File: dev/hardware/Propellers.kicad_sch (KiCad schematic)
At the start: 17 parts, among them J201 CPU PGMR, J202 SPARE CPU HDR, J203 GPU PGMR, J204 SPARE GPU HDR, SW201 CPU ~{RES}, SW202 DEBUG, SW203 GPU ~{RES}

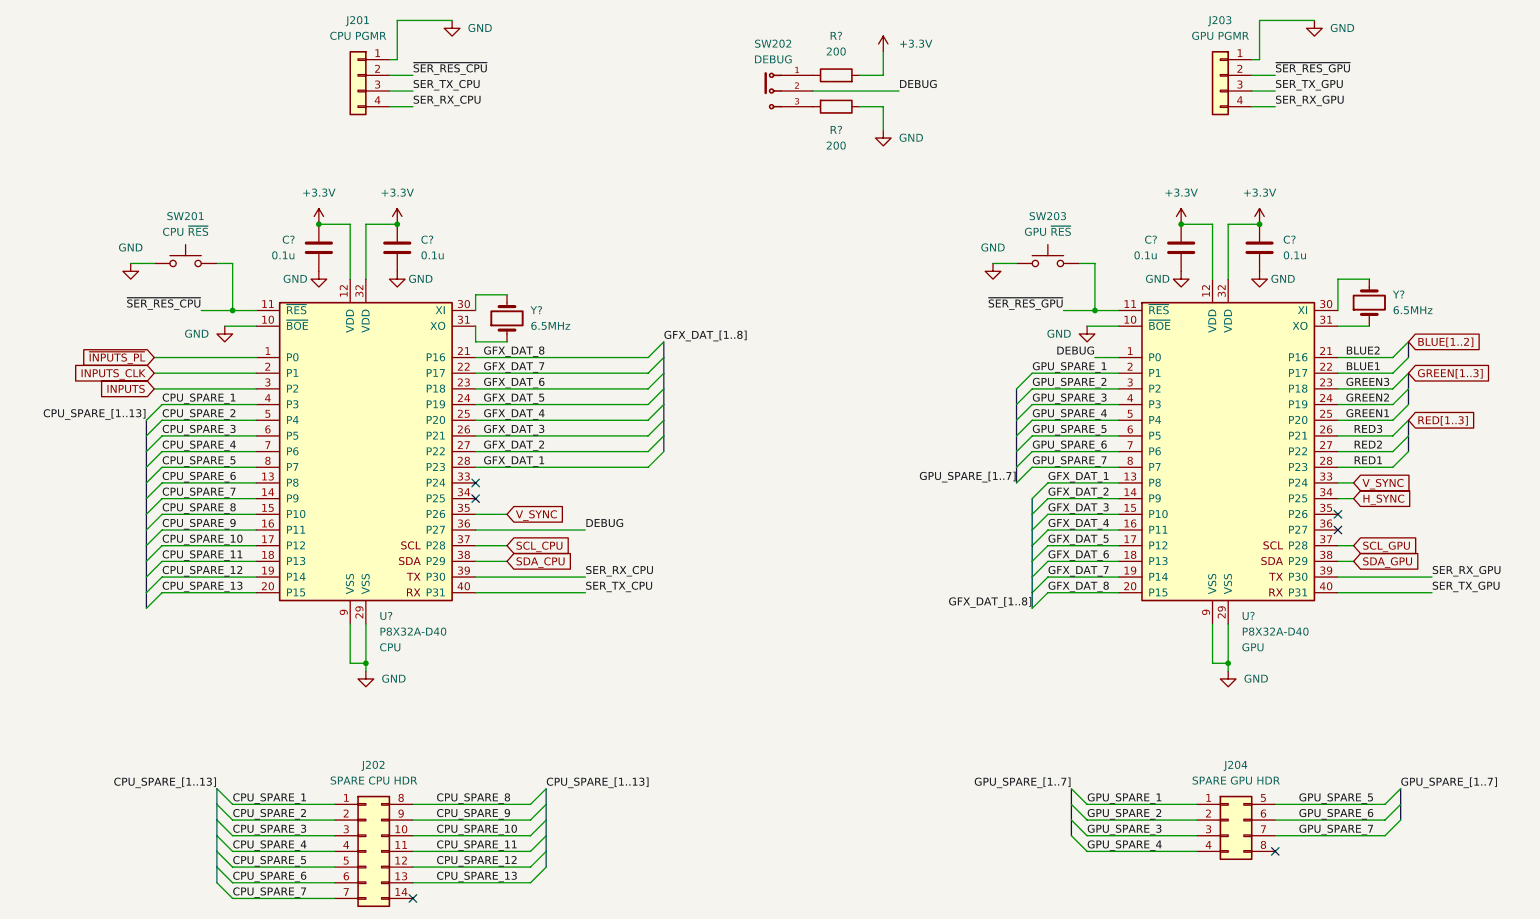
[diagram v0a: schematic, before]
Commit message: Finalized dev board administrivia
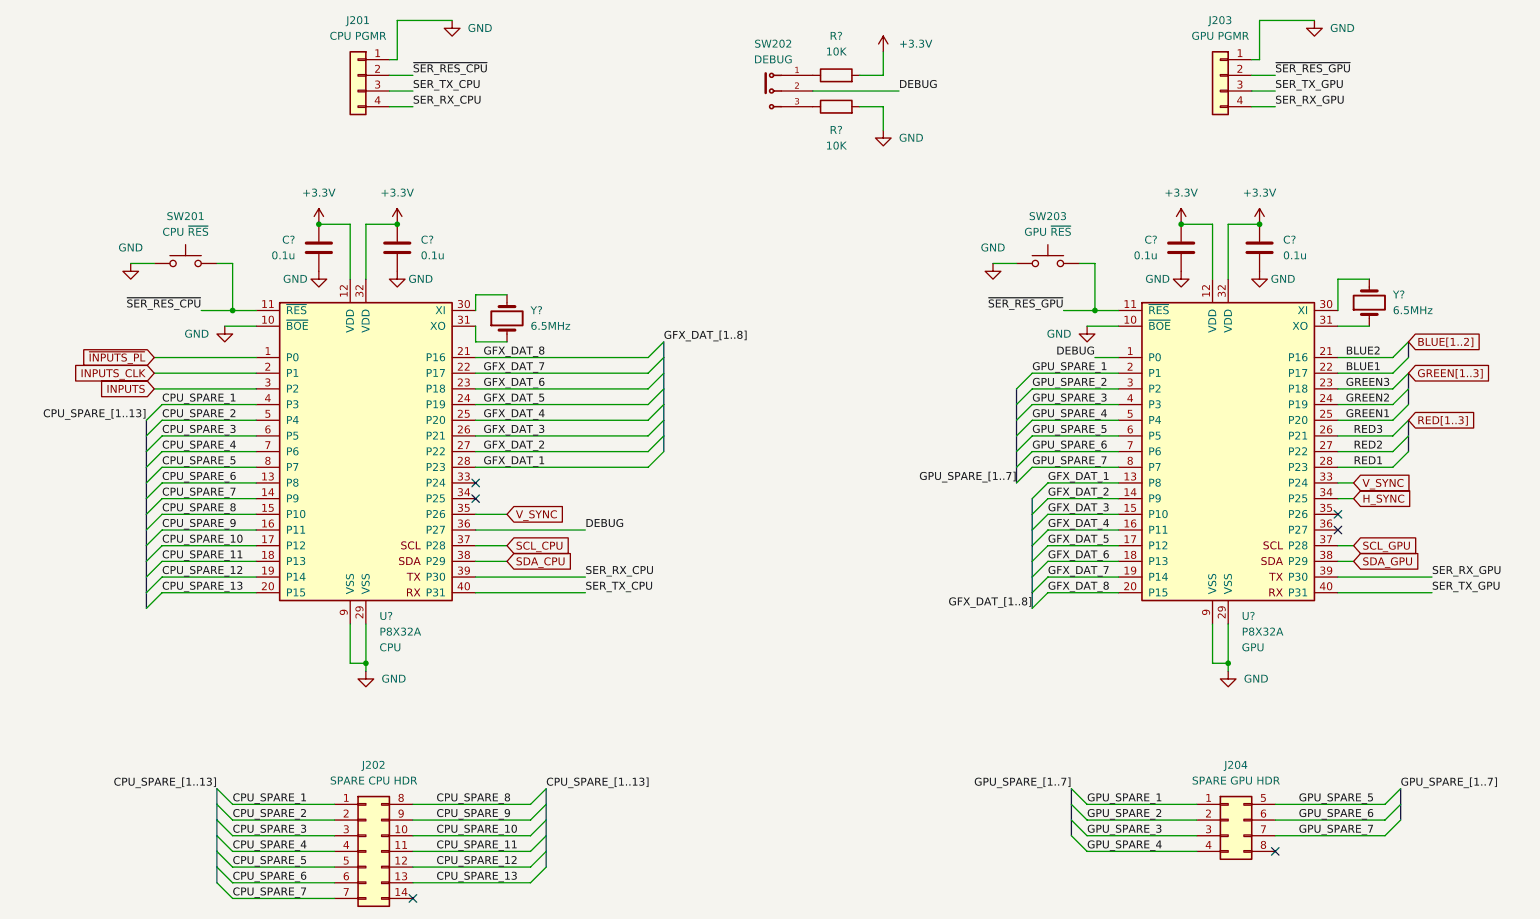
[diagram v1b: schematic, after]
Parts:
- removed C? (x3): 0.1u, Capacitor_THT:C_Disc_D3.4mm_W2.1mm_P2.50mm, symbol Device:C
- removed R?: 200, Resistor_THT:R_Axial_DIN0207_L6.3mm_D2.5mm_P10.16mm_Horizontal, symbol Device:R
- removed Y?: 6.5MHz, Crystal:Crystal_HC49-U_Vertical, symbol Device:Crystal
- added C? (x3): 0.1u, Capacitor_THT:C_Disc_D3.4mm_W2.1mm_P2.50mm, symbol Device:C
- added R?: 10K, Resistor_THT:R_Axial_DIN0207_L6.3mm_D2.5mm_P10.16mm_Horizontal, symbol Device:R
- added Y?: 6.5MHz, Crystal:Crystal_HC49-U_Vertical, symbol Device:Crystal
- C?, J201, J203: Part (none) -> K104K15X7RF5TL2
- J202: Part (none) -> PH2-14-UA
- J204: Part (none) -> PH2-08-UA
- R?: value 200 -> 10K; Part (none) -> RNF14FTD10K0
- SW201, SW203: Part (none) -> B3F-1002
- SW202: Part (none) -> EG1218
- U? (x2): value P8X32A-D40 -> P8X32A; Part (none) -> P8X32A-D40
- Y?: Part (none) -> ECS-65-20-4X
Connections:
- net +3.3V: now also C?.2, C?.2, C?.2
- net GND: now also C?.1, C?.1, C?.1, R?.2
- net at SW202.3: now also R?.1
- net at U?.31 (XO): now also Y?.1
- net at U?.30 (XI): now also Y?.2
